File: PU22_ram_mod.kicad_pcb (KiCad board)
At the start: 2 copper layers, 39.2 x 104.7 mm, 11 parts, among them J1 MOBO, J2 BA8, J3 BA10

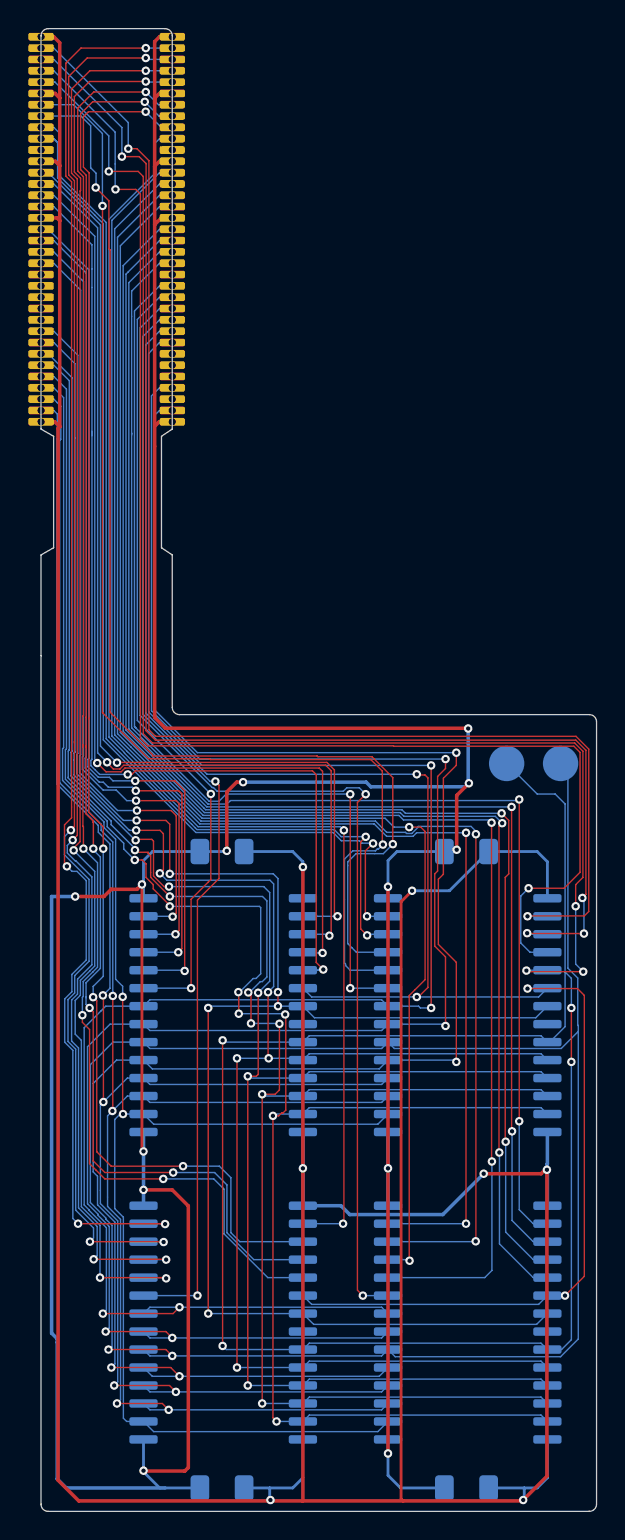
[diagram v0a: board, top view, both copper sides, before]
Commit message: Change outline
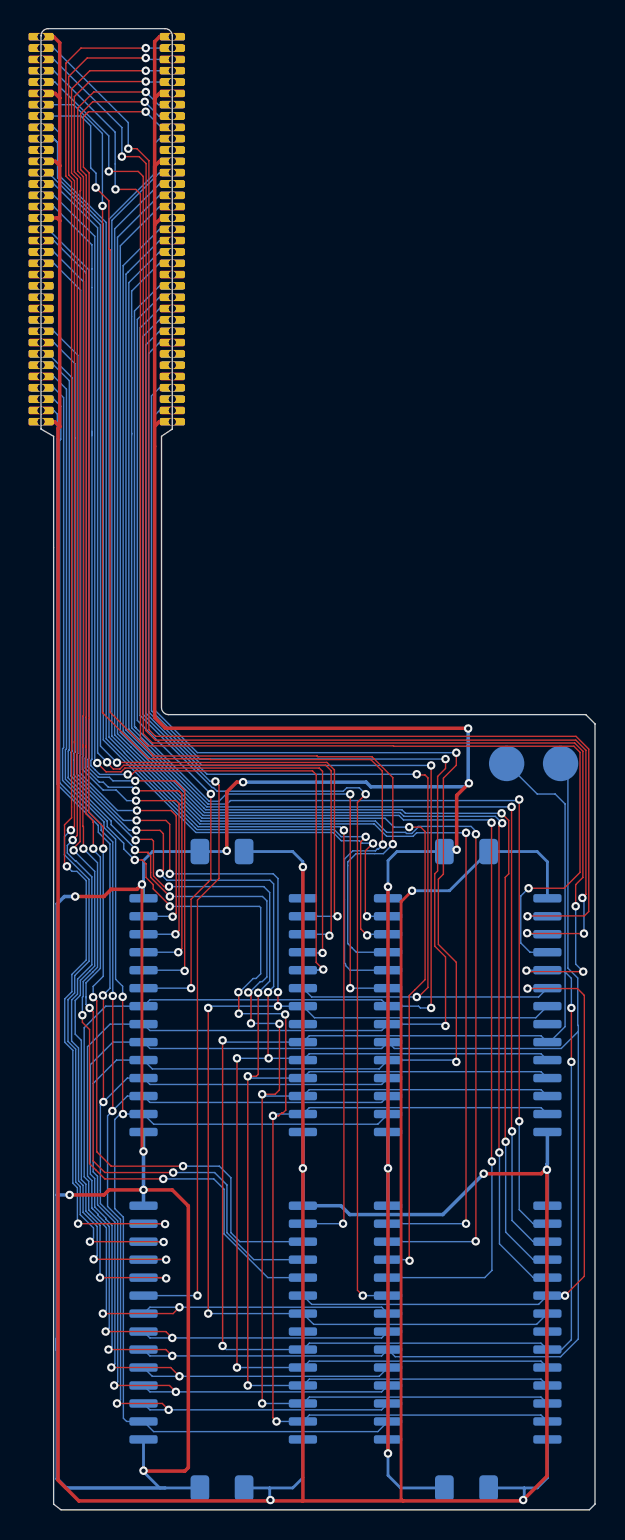
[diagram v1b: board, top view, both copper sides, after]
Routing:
- net GND: track 290.1 -> 296.2 mm, vias 13 -> 14
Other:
- board size 39.2 x 104.7 mm -> 39.1 x 104.6 mm
